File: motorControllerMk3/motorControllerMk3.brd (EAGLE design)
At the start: 61.6 x 54.6 mm, 40 parts, among them IC1 VNH3SP30, IC2 VNH3SP30

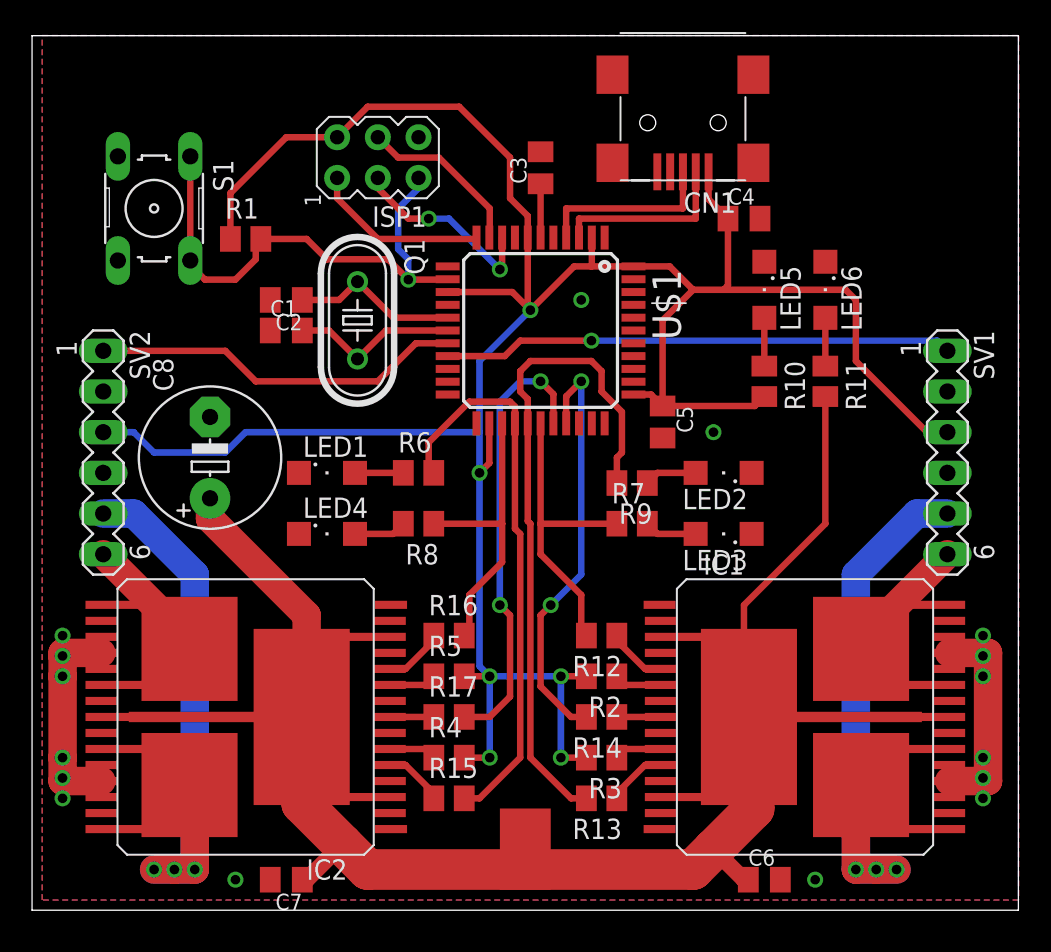
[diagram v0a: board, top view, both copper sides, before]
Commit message: finalizing layout
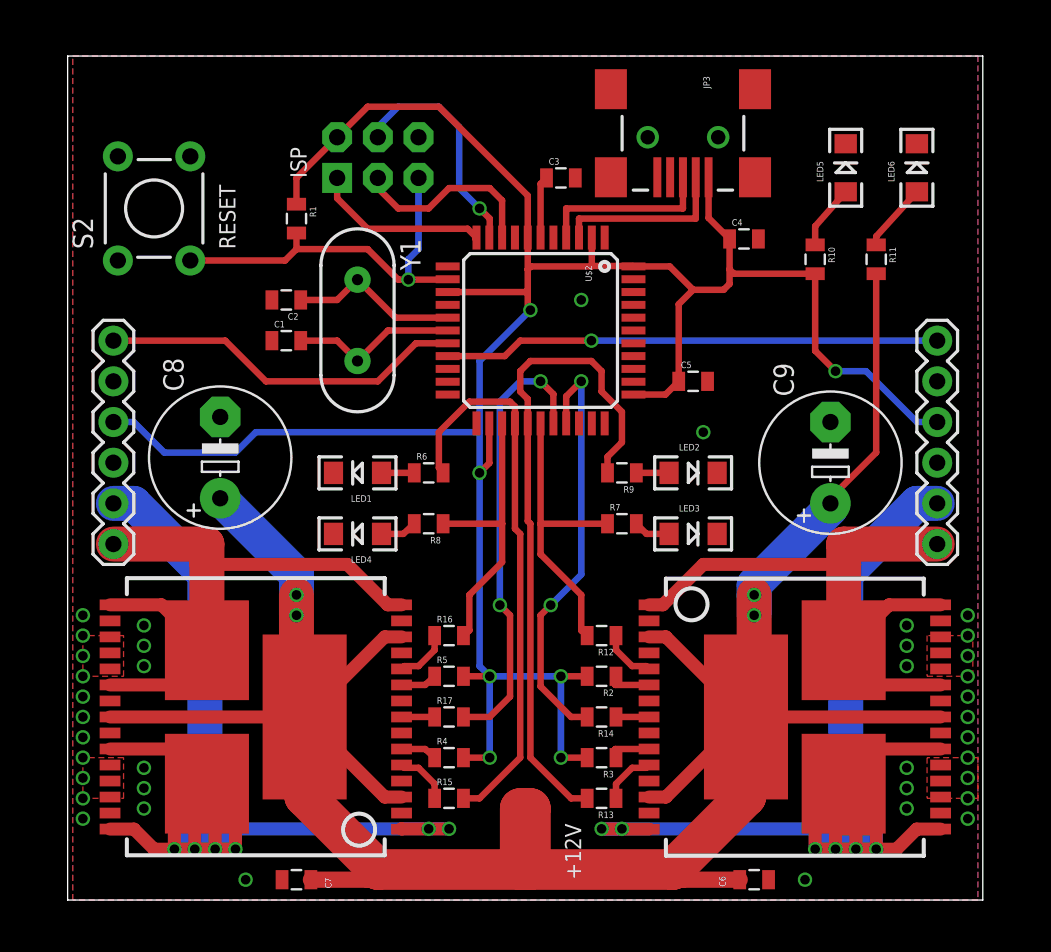
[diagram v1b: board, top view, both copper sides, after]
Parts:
- removed CN1: (no value), adafruit:USB-MINIB
- removed IC1, IC2: VNH3SP30, st-microelectronics:MULTIPOWERSO-30
- removed ISP1: AVRISP-6, adafruit:AVRISP
- removed Q1: (no value), adafruit:HC49U-V
- removed S1: (no value), switch-omron:B3F-10XX
- removed SV1, SV2: (no value), con-lstb:MA06-1
- added C9: 2200u, rcl:E5-8,5
- added J1: AVR_SPI_PRG_6NS, SparkFun-Connectors:2X3-NS
- added JP1, JP2: (no value), SparkFun-Connectors:1X06
- added JP3: USB-SMD-NS, SparkFun-Connectors:USB-MINIB-NOSTOP
- added S2: SWITCH-MOMENTARY-2PTH, SparkFun-Electromechanical:TACTILE-PTH
- added U$2: ATMEGA32U4TQFP, SparkFun-DigitalIC:SPARKFUN-DIGITALIC_TQFP44
- added U$3: VNH2SP30, SparkFun-PowerIC:VNH2SP30
- added Y1: (no value), SparkFun-FreqCtrl:HC49US
- C1, C2, C3, C4, C5, C6, C7: device rcl:C0805K -> SparkFun-Passives:0805
- LED1: value (none) -> A2; device led:SML1206 -> SparkFun-LED:LED-1206
- LED2: value (none) -> B1; device led:SML1206 -> SparkFun-LED:LED-1206
- LED3: value (none) -> A1; device led:SML1206 -> SparkFun-LED:LED-1206
- LED4: value (none) -> B2; device led:SML1206 -> SparkFun-LED:LED-1206
- LED5: value (none) -> +5V; device led:SML1206 -> SparkFun-LED:LED-1206
- LED6: value (none) -> +12V; device led:SML1206 -> SparkFun-LED:LED-1206
- R1: value (none) -> 10k; device rcl:M0805 -> SparkFun-Passives:0805
- R10, R11, R12, R13, R14, R15, R16, R17, R2, R3, R4, R5, R6, R7, R8, R9: device rcl:M0805 -> SparkFun-Passives:0805
- U$1: value ATMEGA32U4-AU -> VNH2SP30; device adafruit:TQFP44 -> SparkFun-PowerIC:VNH2SP30
- moved U$1 30.0 mm to (33.7, 21.6), turned to 90 degrees
- moved LED6 9.53 mm to (74.9, 55.9), turned to 90 degrees
- moved LED5 9.16 mm to (70.5, 55.9), turned to 90 degrees
- moved R10 8.25 mm to (68.6, 50.2)
- moved R11 8.25 mm to (72.4, 50.2)
- moved R1 3.42 mm to (36.2, 52.7), turned to 270 degrees
- moved C5 3.18 mm to (61.0, 42.5), turned to 0 degrees
- moved LED1 1.91 mm to (40.0, 36.8), turned to 180 degrees
- moved LED2 1.91 mm to (61.0, 36.8), turned to 0 degrees
- moved LED3 1.91 mm to (61.0, 33.0), turned to 0 degrees
- moved LED4 1.91 mm to (40.0, 33.0), turned to 180 degrees
- moved C3 1.42 mm to (52.7, 55.2), turned to 0 degrees
- moved C4 1.27 mm to (64.1, 51.4)
- moved R9 0.90 mm to (56.5, 36.8)
- moved C6 0.64 mm to (64.8, 11.4)
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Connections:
- removed net N$14: IC1.15, IC1.16, IC1.21, IC1.OUTB, IC1.OUTB@1, SV1.5
- removed net N$15: IC2.15, IC2.16, IC2.21, IC2.OUTB, IC2.OUTB@1, SV2.6
- removed net N$16: IC2.1, IC2.25, IC2.30, IC2.OUTA, IC2.OUTA@1, SV2.5
- removed net N$18: IC2.6, R4.1
- removed net N$19: IC2.10, R5.1
- removed net N$21: IC1.10, R3.1
- removed net N$23: R16.2, R8.1, U$1.25
- removed net N$24: R12.2, R7.1, U$1.28
- removed net N$25: R15.2, R6.2, U$1.26
- removed net N$26: R13.2, R9.2, U$1.27
- removed net N$32: IC1.5, R12.1
- removed net N$33: IC1.11, R13.1
- removed net N$34: IC1.8, R14.1
- removed net N$35: IC2.5, R15.1
- removed net N$36: IC2.11, R16.1
- removed net N$37: IC2.8, R17.1
- new net N$5: R16.1, U$1.11
- new net OUTA1: JP1.1, U$3.1, U$3.25, U$3.30, U$3.SLUG3
- new net OUTA2: JP2.2, U$1.1, U$1.25, U$1.30, U$1.SLUG3
- new net OUTB1: JP1.2, U$3.15, U$3.16, U$3.21, U$3.SLUG2
- new net OUTB2: JP2.1, U$1.15, U$1.16, U$1.21, U$1.SLUG2
- new net PB0: U$2.8
- new net PB1: J1.3, U$2.9
- new net PB2: J1.4, U$2.10
- new net PB3: J1.1, U$2.11
- new net PB4: R12.2, R7.1, U$2.28
- new net PB5: R17.2, U$2.29
- new net PB6: R14.2, U$2.30
- new net PB7: U$2.12
- new net PC6: U$2.31
- new net PC7: U$2.32
- new net PD0: JP2.6, U$2.18
- new net PD1: JP1.6, U$2.19
- new net PD2: U$2.20
- new net PD3: U$2.21
- new net PD4: R16.2, R8.1, U$2.25
- new net PD5: U$2.22
- new net PD6: R15.2, R6.2, U$2.26
- new net PD7: R13.2, R9.2, U$2.27
- new net PE6: U$2.1
- net +12V: now also C9.+, U$1.13, U$1.23, U$1.3, U$1.SLUG1, U$3.13, U$3.23, U$3.3, U$3.SLUG1; no longer IC1.13, IC1.23, IC1.3, IC1.VCC, IC1.VCC@1, IC2.13, IC2.23, IC2.3, IC2.VCC, IC2.VCC@1
- net +5V: now also J1.2, JP1.4, JP2.4, JP3.VBUS, U$2.14, U$2.2, U$2.24, U$2.34, U$2.44, U$2.7; no longer CN1.VBUS, ISP1.2, SV1.3, SV2.3, U$1.14, U$1.2, U$1.24, U$1.34, U$1.44, U$1.7
- net GND: now also C9.-, J1.6, JP1.3, JP2.3, JP3.GND, S2.1, U$1.18, U$1.19, U$1.20, U$1.26, U$1.27, U$1.28, U$2.15, U$2.23, U$2.35, U$2.43, U$2.5, U$3.18, U$3.19, U$3.20, U$3.26, U$3.27, U$3.28; no longer CN1.GND, IC1.18, IC1.19, IC1.20, IC1.26, IC1.27, IC1.28, IC2.18, IC2.19, IC2.20, IC2.26, IC2.27, IC2.28, ISP1.6, S1.3, S1.4, SV1.4, SV2.4, U$1.15, U$1.23, U$1.35, U$1.43, U$1.5
- net N$1: now also R15.1, U$1.5; no longer ISP1.3, U$1.9
- net N$10: now also JP3.D+, U$2.4; no longer CN1.D+, U$1.4
- net N$11: now also JP3.D-, U$2.3; no longer CN1.D-, U$1.3
- net N$12: now also R13.1, U$3.11; no longer SV2.1, U$1.18
- net N$13: now also R14.1, U$3.8; no longer IC1.1, IC1.25, IC1.30, IC1.OUTA, IC1.OUTA@1, SV1.6
- net N$17: now also R3.1, U$3.10; no longer SV1.1, U$1.19
- net N$2: now also U$2.16, Y1.1; no longer Q1.1, U$1.16
- net N$20: now also U$3.6; no longer IC1.6
- net N$3: now also U$2.17, Y1.2; no longer Q1.2, U$1.17
- net N$38: now also J1.5, S2.3, U$2.13; no longer ISP1.5, S1.1, S1.2, U$1.13
- net N$4: now also U$2.6; no longer U$1.6
- net N$6: now also R17.1, U$1.8; no longer ISP1.4, U$1.10
- net N$7: now also R5.1, U$1.10; no longer ISP1.1, U$1.11
- net N$8: now also R4.1, U$1.6; no longer R17.2, U$1.29
- net N$9: now also R12.1, U$3.5; no longer R14.2, U$1.30
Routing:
- net OUTA2: track 0.00 -> 85.4 mm, vias 0 -> 6
- net OUTB1: track 0.00 -> 83.7 mm, vias 0 -> 6
- net +12V: track 87.7 -> 166.6 mm, vias 0 -> 4
- net N$26: track 42.2 -> 0.00 mm
- net PD7: track 0.00 -> 41.8 mm
- net OUTB2: track 0.00 -> 39.9 mm
- net OUTA1: track 0.00 -> 39.9 mm
- net N$14: track 36.2 -> 0.00 mm, vias 3 -> 0
- net N$16: track 36.2 -> 0.00 mm, vias 3 -> 0
- net N$25: track 35.2 -> 0.00 mm
- net PD6: track 0.00 -> 35.0 mm
- net PD1: track 0.00 -> 31.0 mm, vias 0 -> 1
- net N$17: track 31.9 -> 2.65 mm, vias 1 -> 0
- net PB5: track 0.00 -> 28.1 mm, vias 0 -> 2
- net PB6: track 0.00 -> 26.8 mm, vias 0 -> 2
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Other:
- board size 61.6 x 54.6 mm -> 57.1 x 52.7 mm
- board text added: "+12V"
- board text added: "GND"
- board text added: "ISP"
- board text added: "RESET"
